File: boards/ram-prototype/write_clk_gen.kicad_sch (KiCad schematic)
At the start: 24 parts, among them U1 74LVC1G00, U2 74LVC1G00, U3 74LVC1G00, U4 74LVC1G00, U5 74LVC1G00, U6 74LVC1G00, U7 74LVC1G00, U8 74LVC1G00

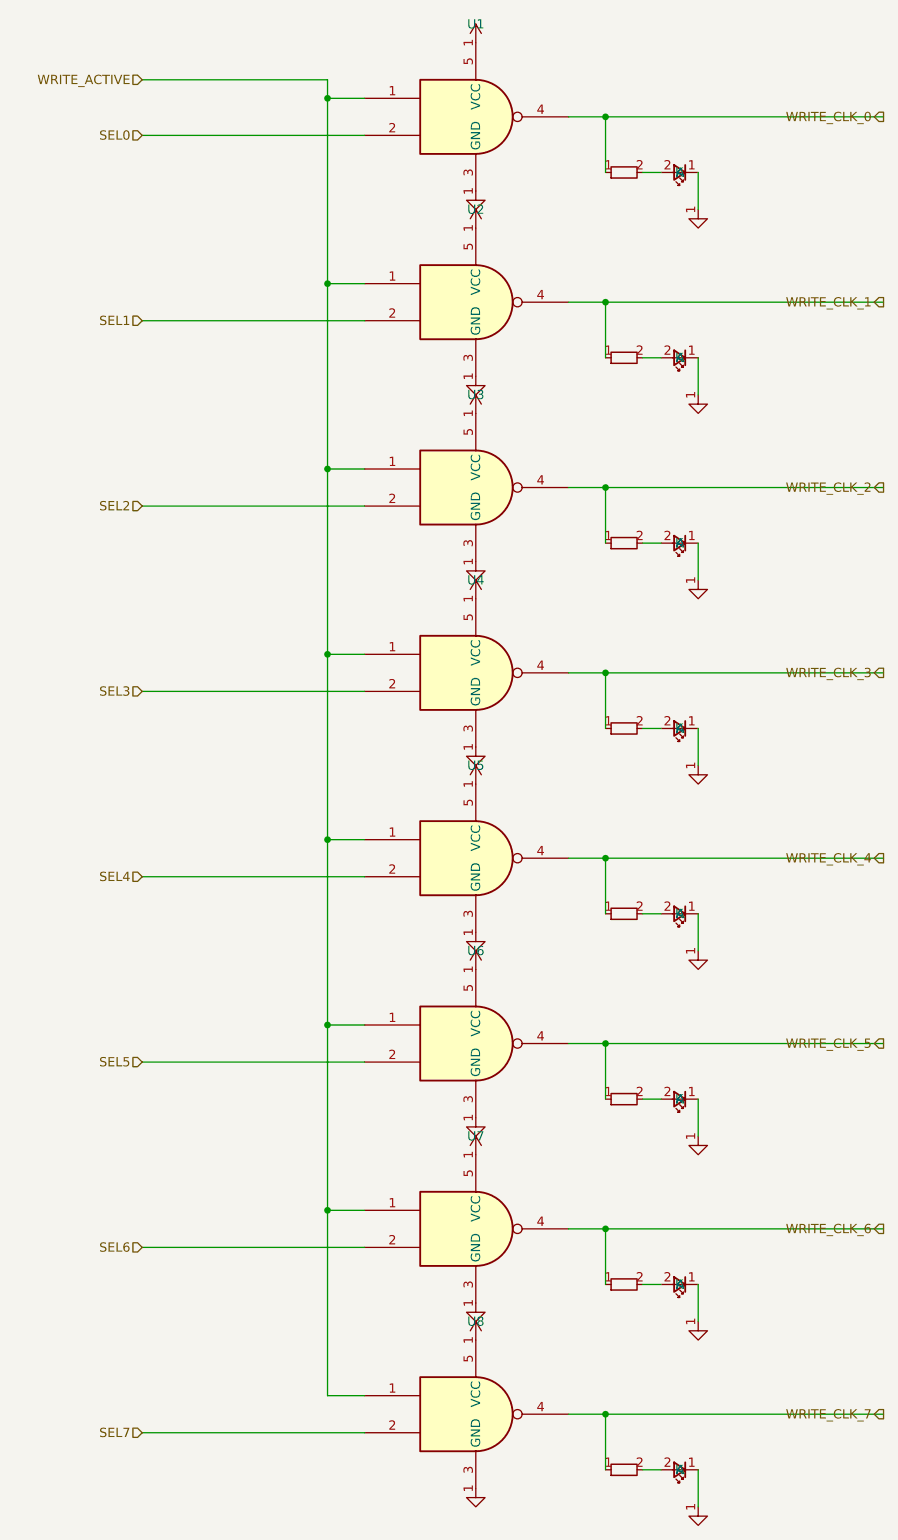
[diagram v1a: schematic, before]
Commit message: Clean up root
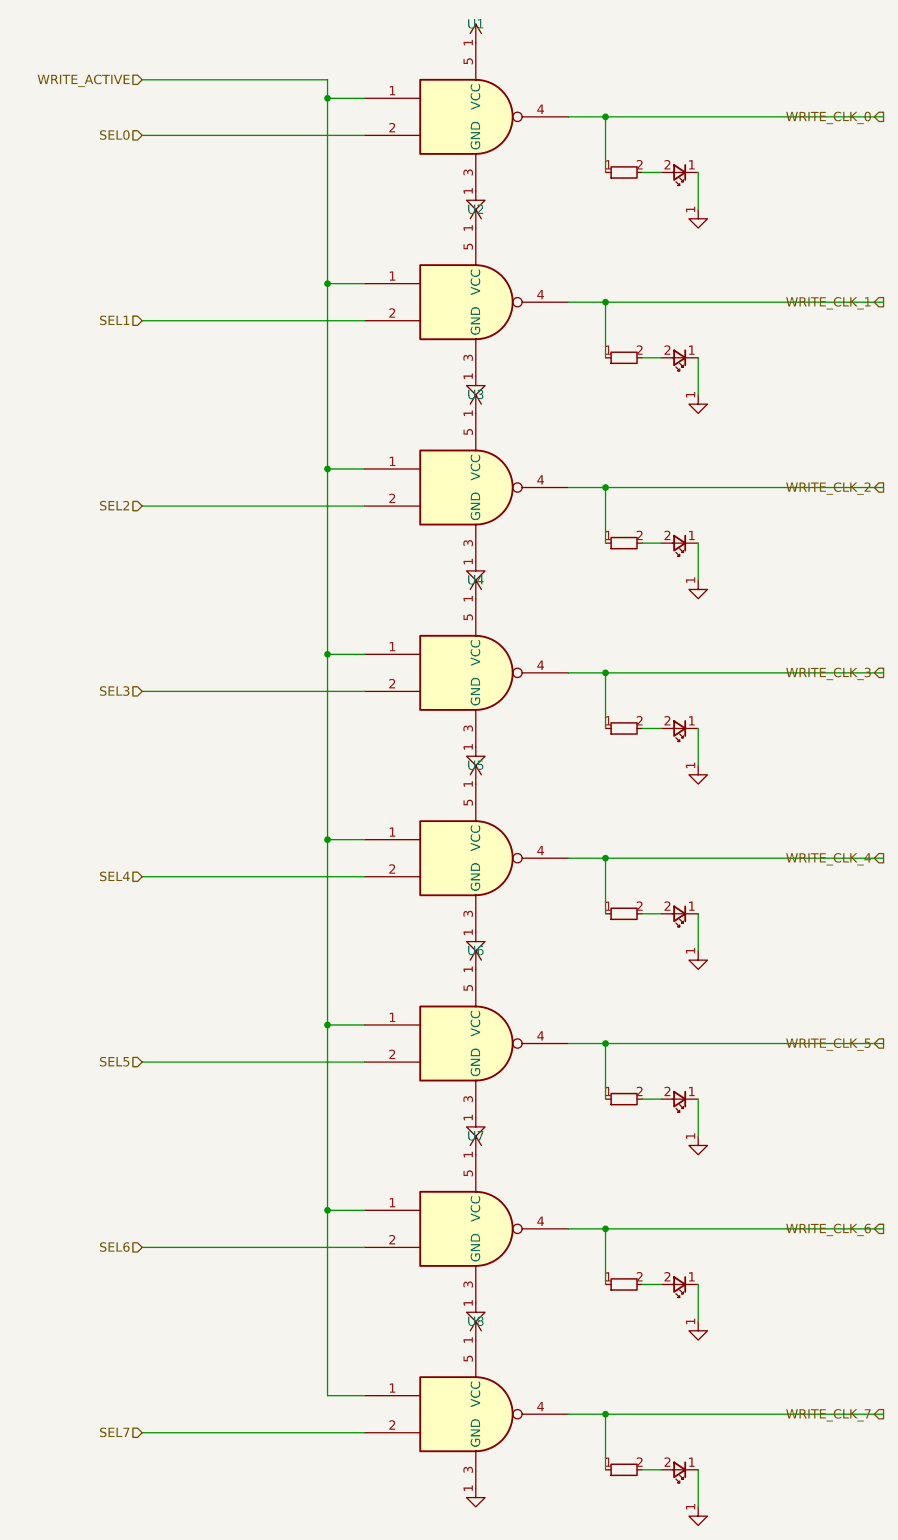
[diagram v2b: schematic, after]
